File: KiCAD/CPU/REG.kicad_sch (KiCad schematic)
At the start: 2 parts, among them U7 74LS374, U8 74LS374

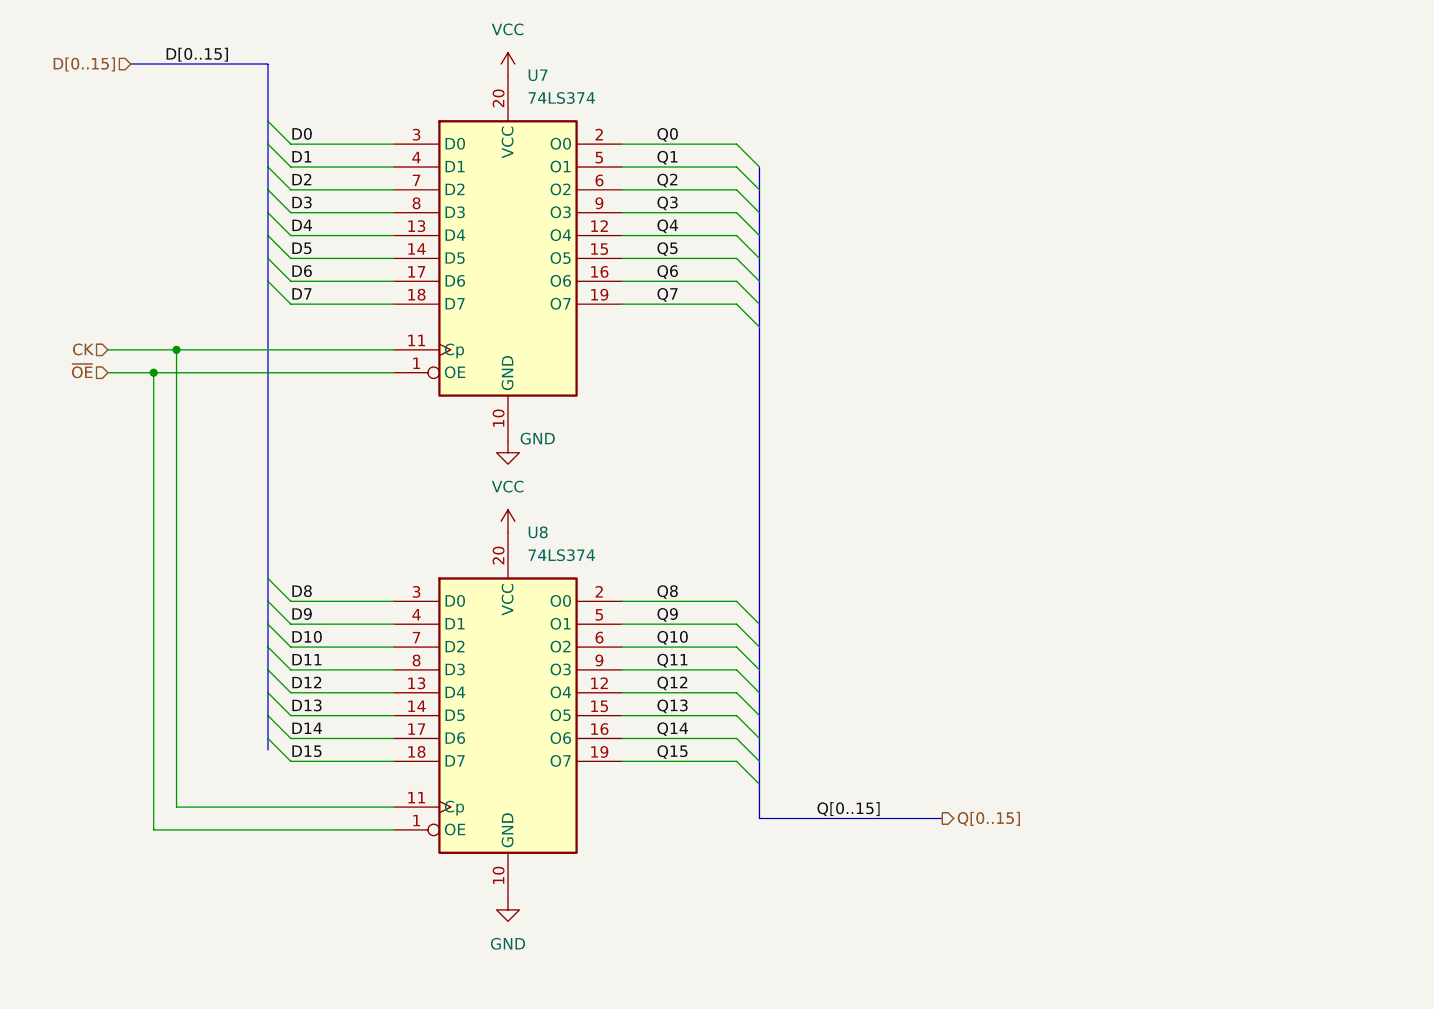
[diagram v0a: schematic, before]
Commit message: small updates
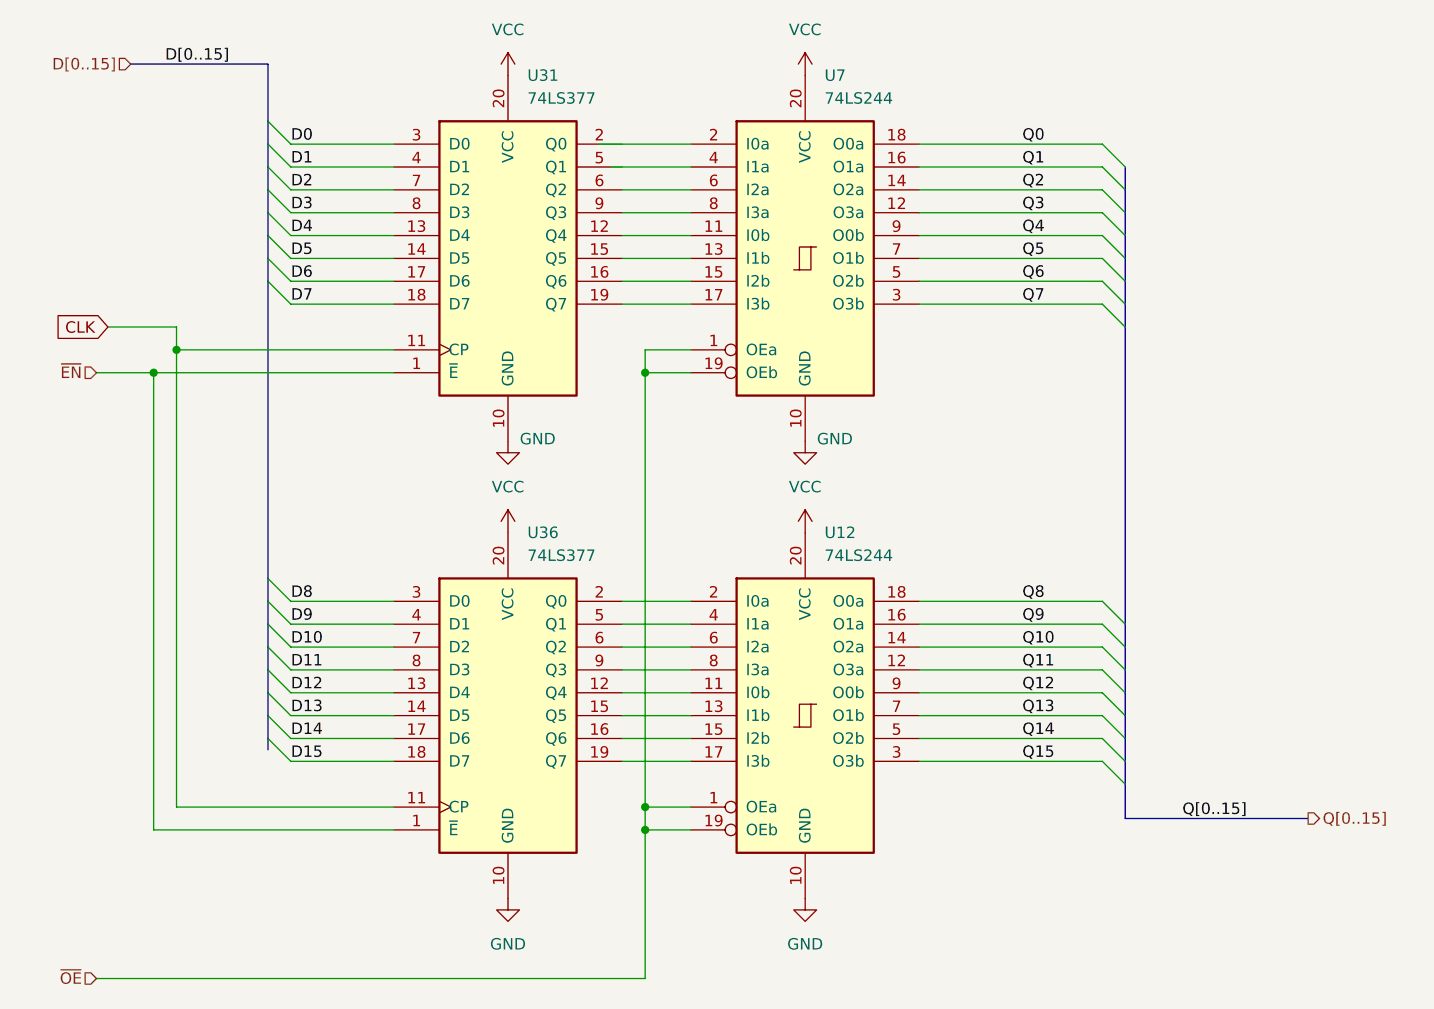
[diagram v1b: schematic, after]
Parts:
- removed U7, U8: 74LS374, symbol 74xx:74LS374
- added U12, U7: 74LS244, symbol 74xx:74LS244
- added U31, U36: 74LS377, symbol 74xx:74LS377
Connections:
- net D0: now also U31.3 (D0)
- net D1: now also U31.4 (D1)
- net D10: now also U36.7 (D2)
- net D11: now also U36.8 (D3)
- net D12: now also U36.13 (D4)
- net D13: now also U36.14 (D5)
- net D14: now also U36.17 (D6)
- net D15: now also U36.18 (D7)
- net D2: now also U31.7 (D2)
- net D3: now also U31.8 (D3)
- net D4: now also U31.13 (D4)
- net D5: now also U31.14 (D5)
- net D6: now also U31.17 (D6)
- net D7: now also U31.18 (D7)
- net D8: now also U36.3 (D0)
- net D9: now also U36.4 (D1)
- net GND: now also U12.10 (GND), U31.10 (GND), U36.10 (GND), U7.10 (GND)
- net Q0: now also U7.18 (O0a)
- net Q1: now also U7.16 (O1a)
- net Q10: now also U12.14 (O2a)
- net Q11: now also U12.12 (O3a)
- net Q12: now also U12.9 (O0b)
- net Q13: now also U12.7 (O1b)
- net Q14: now also U12.5 (O2b)
- net Q15: now also U12.3 (O3b)
- net Q2: now also U7.14 (O2a)
- net Q3: now also U7.12 (O3a)
- net Q4: now also U7.9 (O0b)
- net Q5: now also U7.7 (O1b)
- net Q6: now also U7.5 (O2b)
- net Q7: now also U7.3 (O3b)
- net Q8: now also U12.18 (O0a)
- net Q9: now also U12.16 (O1a)
- net VCC: now also U12.20 (VCC), U31.20 (VCC), U36.20 (VCC), U7.20 (VCC)
- net ~{OE}: now also U12.1 (OEa), U12.19 (OEb), U7.1 (OEa), U7.19 (OEb)
- new net: U12.11 (I0b), U36.12 (Q4)
- new net: U12.13 (I1b), U36.15 (Q5)
- new net: U12.15 (I2b), U36.16 (Q6)
- new net: U12.17 (I3b), U36.19 (Q7)
- new net: U12.2 (I0a), U36.2 (Q0)
- new net: U12.4 (I1a), U36.5 (Q1)
- new net: U12.6 (I2a), U36.6 (Q2)
- new net: U12.8 (I3a), U36.9 (Q3)
- new net: U31.12 (Q4), U7.11 (I0b)
- new net: U31.15 (Q5), U7.13 (I1b)
- new net: U31.16 (Q6), U7.15 (I2b)
- new net: U31.19 (Q7), U7.17 (I3b)
- new net: U31.6 (Q2), U7.6 (I2a)
- new net: U31.9 (Q3), U7.8 (I3a)
- new net CLK: U31.11 (CP), U36.11 (CP)
- new net ~{EN}: U31.1 (~{E}), U36.1 (~{E})
